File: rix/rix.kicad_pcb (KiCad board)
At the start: 2 copper layers, 55 x 30 mm, 20 parts, among them J1 9V BAT - +, J2 Detection coil, J3 External antenna, SW1 On/Off SW, U1 74LS04, U2 L78L05_SOT89, Y1 8.0 Mhz Crystal, Y2 8.0 Mhz Crystal

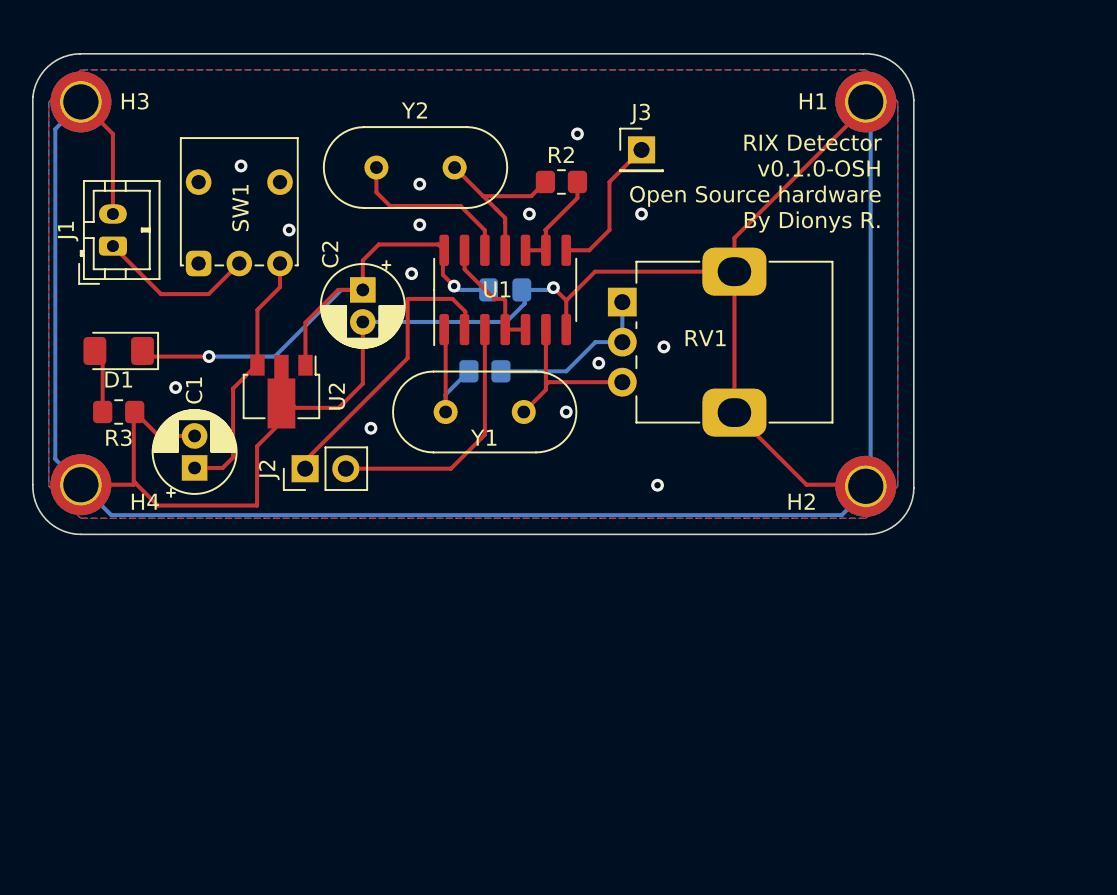
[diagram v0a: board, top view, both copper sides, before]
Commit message: Updating gerber files
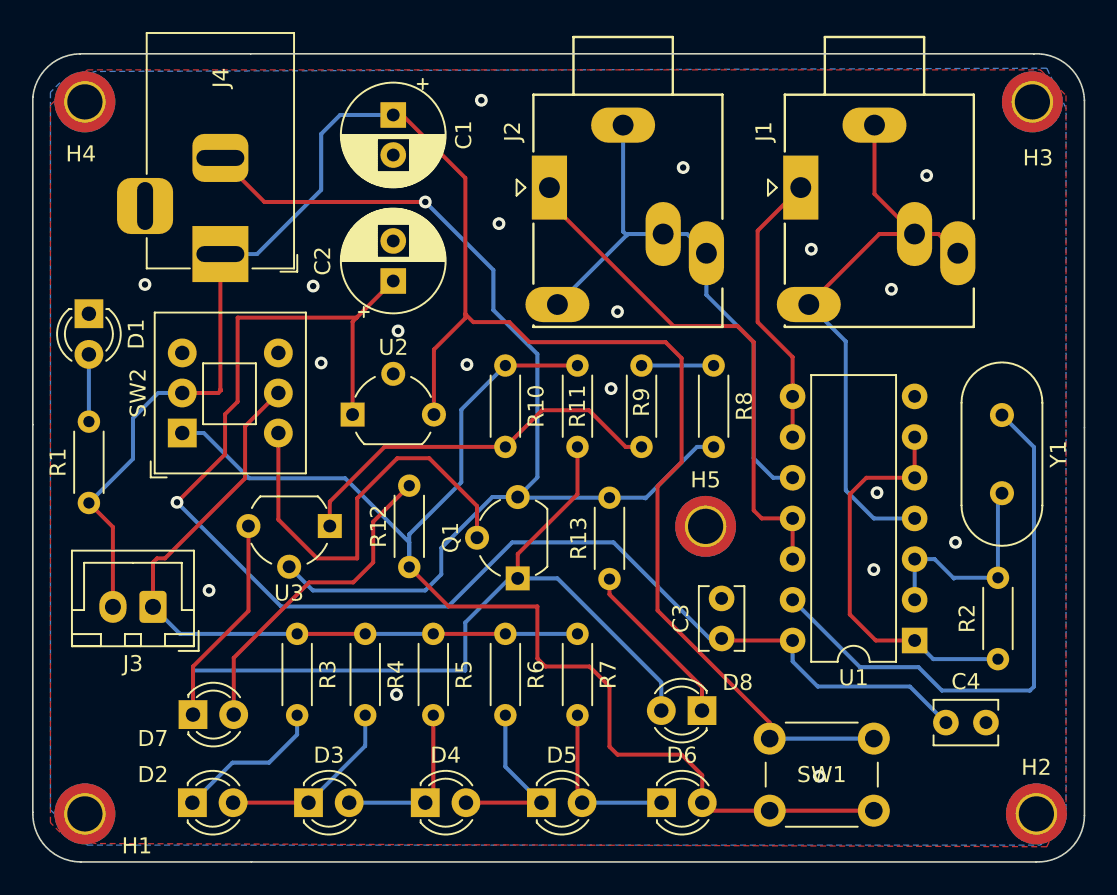
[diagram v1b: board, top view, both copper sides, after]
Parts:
- removed RV1: 10K tunnig POT, Potentiometer_THT:Potentiometer_Alps_RK09K_Single_Vertical
- removed Y2: 8.0 Mhz Crystal, Crystal:Crystal_HC49-4H_Vertical
- added C4: C_Small, Capacitor_THT:C_Disc_D3.8mm_W2.6mm_P2.50mm, F.Cu at (138.0, 105.8)
- added D2: LED, LED_THT:LED_D3.0mm, F.Cu at (91.0, 110.8)
- added D3: LED, LED_THT:LED_D3.0mm, F.Cu at (98.2, 110.8)
- added D4: LED, LED_THT:LED_D3.0mm, F.Cu at (105.5, 110.8)
- added D5: LED, LED_THT:LED_D3.0mm, F.Cu at (112.8, 110.8)
- added D6: LED, LED_THT:LED_D3.0mm, F.Cu at (120.2, 110.8)
- added D7: LED, LED_THT:LED_D3.0mm, F.Cu at (91.0, 105.2)
- added D8: LED, LED_THT:LED_D3.0mm, F.Cu at (122.8, 105.0)
- added H5: MountingHole_Pad, MountingHole:MountingHole_2.2mm_M2_DIN965_Pad_TopBottom, F.Cu at (123.0, 93.5)
- added J4: Barrel_Jack_Switch, Connector_BarrelJack:BarrelJack_Horizontal, F.Cu at (92.7, 76.5)
- added Q1: IRFS4127, Package_TO_SOT_THT:TO-92_Wide, F.Cu at (111.3, 96.8)
- added R10: R, Resistor_THT:R_Axial_DIN0204_L3.6mm_D1.6mm_P5.08mm_Horizontal, F.Cu at (110.5, 83.5)
- added R11: R, Resistor_THT:R_Axial_DIN0204_L3.6mm_D1.6mm_P5.08mm_Horizontal, F.Cu at (115.0, 83.5)
- added R12: R, Resistor_THT:R_Axial_DIN0204_L3.6mm_D1.6mm_P5.08mm_Horizontal, F.Cu at (104.5, 96.0)
- added R13: R, Resistor_THT:R_Axial_DIN0204_L3.6mm_D1.6mm_P5.08mm_Horizontal, F.Cu at (117.0, 96.8)
- added R4: R, Resistor_THT:R_Axial_DIN0204_L3.6mm_D1.6mm_P5.08mm_Horizontal, F.Cu at (101.8, 100.2)
- added R5: R, Resistor_THT:R_Axial_DIN0204_L3.6mm_D1.6mm_P5.08mm_Horizontal, F.Cu at (106.0, 100.2)
- added R6: R, Resistor_THT:R_Axial_DIN0204_L3.6mm_D1.6mm_P5.08mm_Horizontal, F.Cu at (110.5, 100.2)
- added R7: R, Resistor_THT:R_Axial_DIN0204_L3.6mm_D1.6mm_P5.08mm_Horizontal, F.Cu at (115.0, 100.2)
- added R8: R, Resistor_THT:R_Axial_DIN0204_L3.6mm_D1.6mm_P5.08mm_Horizontal, F.Cu at (123.5, 83.5)
- added R9: R, Resistor_THT:R_Axial_DIN0204_L3.6mm_D1.6mm_P5.08mm_Horizontal, F.Cu at (119.0, 88.5)
- added SW2: SW_Push_DPDT, Button_Switch_THT:SW_Push_2P2T_Toggle_CK_PVA2OAH5xxxxxxV2, F.Cu at (90.3, 87.7)
- added U3: TL431PK, Package_TO_SOT_THT:TO-92_Wide, F.Cu at (99.5, 93.5)
- C1: value 50v 10uF -> C_Polarized; footprint Capacitor_THT:CP_Radial_D5.0mm_P2.00mm -> Capacitor_THT:CP_Radial_D6.3mm_P2.50mm
- C2: value 50v 1uF -> C_Polarized; footprint Capacitor_THT:CP_Radial_D5.0mm_P2.00mm -> Capacitor_THT:CP_Radial_D6.3mm_P2.50mm
- C3: value 10nF -> C_Small; footprint Capacitor_SMD:C_0805_2012Metric_Pad1.18x1.45mm_HandSolder -> Capacitor_THT:C_Disc_D3.8mm_W2.6mm_P2.50mm; moved to F.Cu
- D1: footprint Diode_SMD:D_1206_3216Metric_Pad1.42x1.75mm_HandSolder -> LED_THT:LED_D3.0mm
- J1: value 9V BAT - + -> AudioJack3_SwitchTR; footprint Connector_JST:JST_PH_B2B-PH-K_1x02_P2.00mm_Vertical -> Connector_Audio:Jack_3.5mm_Ledino_KB3SPRS_Horizontal
- J2: value Detection coil -> AudioJack3_SwitchTR; footprint Connector_PinHeader_2.54mm:PinHeader_1x02_P2.54mm_Vertical -> Connector_Audio:Jack_3.5mm_Ledino_KB3SPRS_Horizontal
- J3: value External antenna -> Conn_01x02_Male; footprint Connector_PinHeader_2.54mm:PinHeader_1x01_P2.54mm_Vertical -> Connector_JST:JST_XH_B2B-XH-A_1x02_P2.50mm_Vertical
- R1: value 1M -> R; footprint Resistor_SMD:R_0805_2012Metric_Pad1.20x1.40mm_HandSolder -> Resistor_THT:R_Axial_DIN0204_L3.6mm_D1.6mm_P5.08mm_Horizontal; moved to F.Cu
- R2: value 1K -> R; footprint Resistor_SMD:R_0805_2012Metric_Pad1.20x1.40mm_HandSolder -> Resistor_THT:R_Axial_DIN0204_L3.6mm_D1.6mm_P5.08mm_Horizontal
- R3: value 220R -> R; footprint Resistor_SMD:R_0805_2012Metric_Pad1.20x1.40mm_HandSolder -> Resistor_THT:R_Axial_DIN0204_L3.6mm_D1.6mm_P5.08mm_Horizontal
- SW1: value On/Off SW -> SW_DIP_x01; footprint Button_Switch_THT:SW_Push_1P2T_Vertical_E-Switch_800UDP8P1A1M6 -> Button_Switch_THT:SW_PUSH_6mm_H5mm
- U1: value 74LS04 -> 74LS02; footprint Package_SO:SOIC-14_3.9x8.7mm_P1.27mm -> Package_DIP:DIP-14_W7.62mm
- U2: value L78L05_SOT89 -> L78L05_TO92; footprint Package_TO_SOT_SMD:SOT-89-3 -> Package_TO_SOT_THT:TO-92_Wide
- Y1: value 8.0 Mhz Crystal -> Crystal
- moved H1 66.0 mm to (84.2, 111.5)
- moved H3 59.4 mm to (143.4, 67.0)
- moved SW1 54.3 mm to (133.5, 111.2), turned to 180 degrees
- moved J1 43.1 mm to (128.9, 72.3), turned to -90 degrees
- moved J3 41.8 mm to (88.5, 98.5), turned to 180 degrees
- moved R2 40.4 mm to (141.2, 101.8), turned to 90 degrees
- moved Y1 34.7 mm to (141.5, 86.5), turned to -90 degrees
- moved U1 33.6 mm to (136.1, 100.6), turned to 180 degrees
- moved R1 26.1 mm to (84.5, 92.0), turned to 90 degrees
- moved C3 25.6 mm to (124.0, 100.5), turned to 90 degrees
- moved C1 25.3 mm to (103.5, 67.8), turned to -90 degrees
- moved H4 23.9 mm to (84.2, 67.0)
- moved J2 23.3 mm to (113.2, 72.3), turned to -90 degrees
- moved H2 23.1 mm to (143.7, 111.5)
- moved R3 17.8 mm to (97.5, 100.2), turned to -90 degrees
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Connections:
- C1 pad 1: Net-(C1-Pad1) -> +9V
- D1 pad 1: Net-(C2-Pad1) -> GND
- R1 pad 1: Net-(R1-Pad1) -> +9V
- R1 pad 2: Net-(R1-Pad2) -> Net-(D1-Pad2)
- R3 pad 1: GND -> Net-(J3-Pad1)
- R3 pad 2: Net-(D1-Pad2) -> Net-(D2-Pad1)
- SW1 pad 1: unconnected-(SW1-Pad1) -> Net-(D6-Pad2)
- SW1 pad 2: Net-(J1-Pad1) -> +9V
- U1 pad 1: Net-(R1-Pad1) -> Net-(R2-Pad1)
- U1 pad 10: Net-(R2-Pad2) -> Net-(J2-PadR)
- U1 pad 11: Net-(R2-Pad1) -> Net-(J2-PadT)
- U1 pad 12: Net-(U1-Pad12) -> Net-(J2-PadT)
- U1 pad 13: IF -> Net-(U1-Pad13)
- U1 pad 2: Net-(J2-Pad1) -> Net-(R2-Pad2)
- U1 pad 3: Net-(J2-Pad2) -> Net-(R2-Pad2)
- U1 pad 4: IF -> Net-(J1-PadR)
- U1 pad 5: IF -> Net-(R2-Pad1)
- U1 pad 6: Net-(RV1-Pad3) -> Net-(R2-Pad1)
- U1 pad 8: Net-(J3-Pad1) -> Net-(J1-PadT)
- U1 pad 9: Net-(R2-Pad2) -> Net-(J1-PadT)
- U2 pad 3: Net-(C1-Pad1) -> +9V
- Y1 pad 1: Net-(R1-Pad1) -> Net-(U1-Pad13)
- Y1 pad 2: Net-(RV1-Pad3) -> Net-(R2-Pad2)
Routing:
- net GND: track 210.5 -> 0.00 mm, vias 15 -> 19
- net +9V: track 0.00 -> 114.8 mm
- net Net-(D6-Pad2): track 0.00 -> 78.5 mm
- net Net-(J4-Pad2): track 0.00 -> 67.6 mm, vias 0 -> 1
- net Net-(D7-Pad1): track 0.00 -> 63.5 mm
- net Net-(C2-Pad1): track 35.0 -> 87.7 mm, vias 2 -> 1
- net Net-(J1-PadR): track 0.00 -> 37.0 mm
- net Net-(J2-PadR): track 0.00 -> 35.5 mm
- net Net-(U1-Pad13): track 0.00 -> 35.3 mm
- net Net-(J3-Pad1): track 9.05 -> 44.1 mm
- net Net-(J2-PadT): track 0.00 -> 33.0 mm
- net Net-(Q1-Pad2): track 0.00 -> 26.8 mm
- net Net-(R10-Pad2): track 0.00 -> 24.3 mm
- net Net-(D7-Pad2): track 0.00 -> 20.4 mm
- net Net-(J2-Pad1): track 18.3 -> 0.00 mm
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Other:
- board size 55 x 30 mm -> 65.7 x 50.5 mm
- board text removed: "RIX Detector v0.1.0-OSH Open Source hardware By Dionys R."
